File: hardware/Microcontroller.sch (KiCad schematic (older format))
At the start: 14 parts, among them J601 SWD, SW601 SW_Push, SW602 SW_Push, U1 BT832, Y601 32kHz

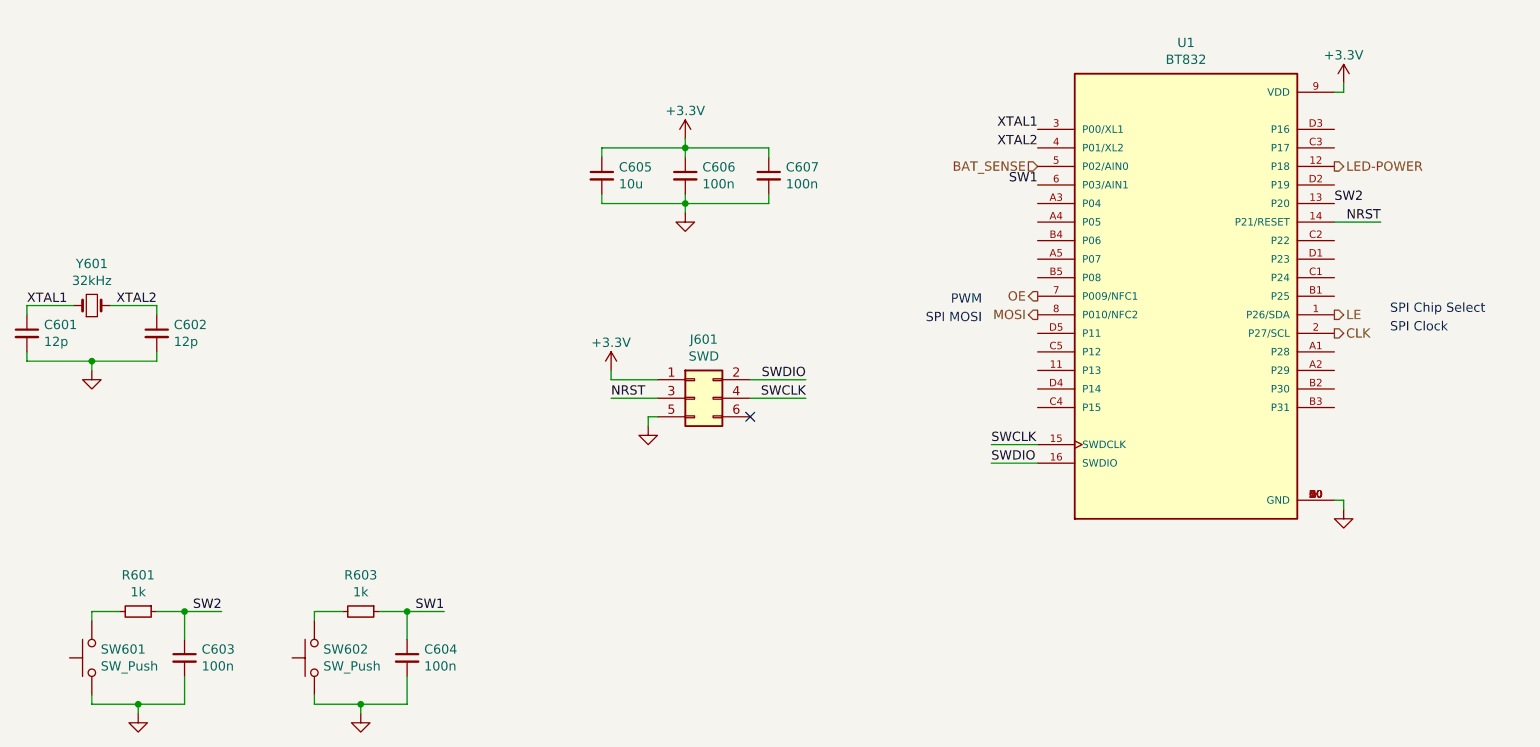
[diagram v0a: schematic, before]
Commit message: Updated to KiCad v6.0
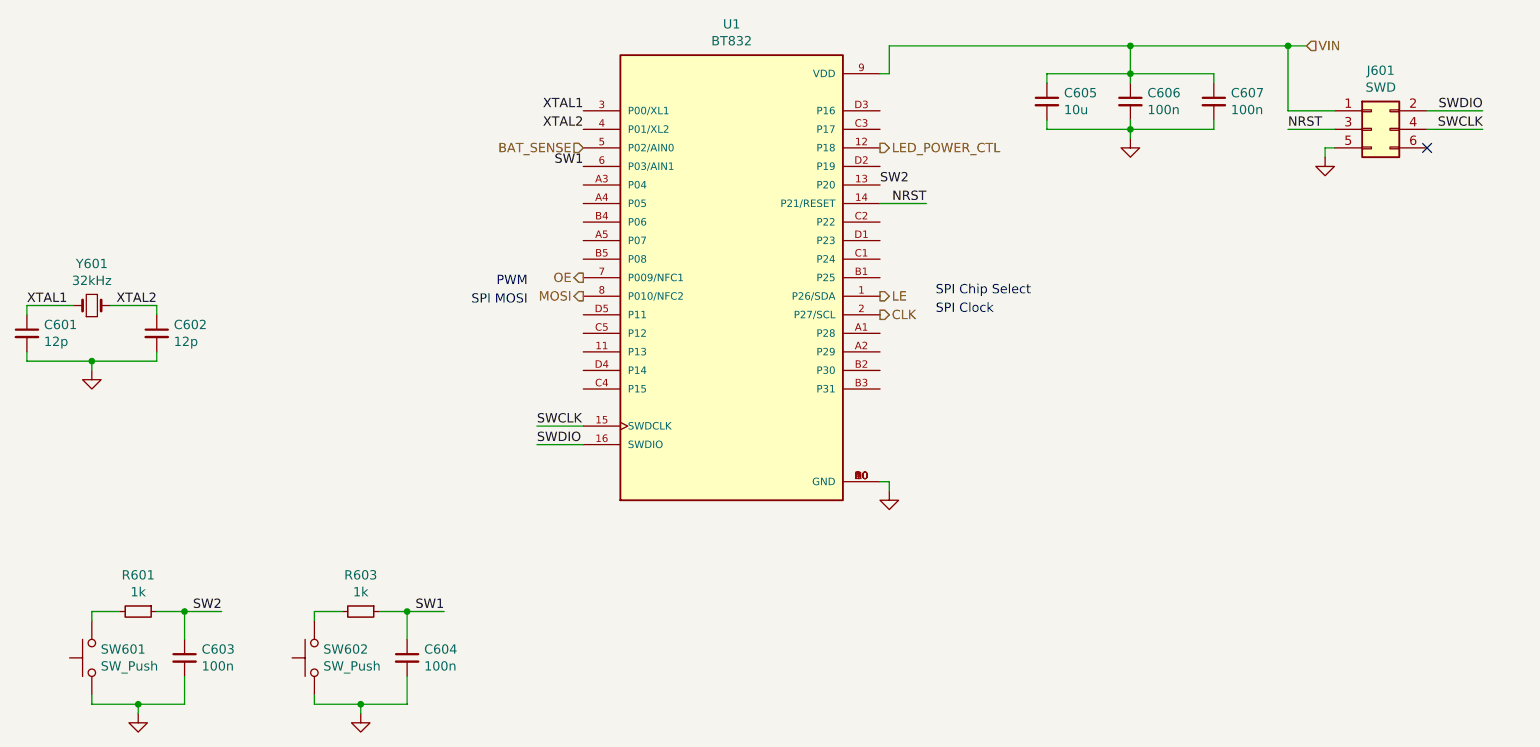
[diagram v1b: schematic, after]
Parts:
- SW601, SW602: MNR KMR211GLFS -> TAC-35N-V-T/R; Manufacturer C&K -> Diptronics; Order https://www.mouser.at/ProductDetail/611-KMR211G-LFS -> https://www.mouser.at/ProductDetail/Diptronics/TAC-35N-V-T-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
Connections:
- net +3V3 renamed VIN
- net LED-POWER renamed LED_POWER_CTL
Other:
- moved on the sheet: C605, C606, C607, J601, U1
